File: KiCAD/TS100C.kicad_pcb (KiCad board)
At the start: 4 copper layers, 84 x 10 mm, 63 parts, among them J1 USB_C_Receptacle_USB2.0, J2 OLED_64x32, J3 A, J4 B, J5 DNP, P1 TC2030-CTX, Q1 SS8050, Q2 DMP3017SFG, SW1 key1, SW2 key2, U1 USBLC6-4SC6, U2 AP2204R-3.3, U3 STUSB4500, U4 STM32F072C8Ux, U5 OPA340NA, U6 MCP9700AT-ETT, U7 SI8540

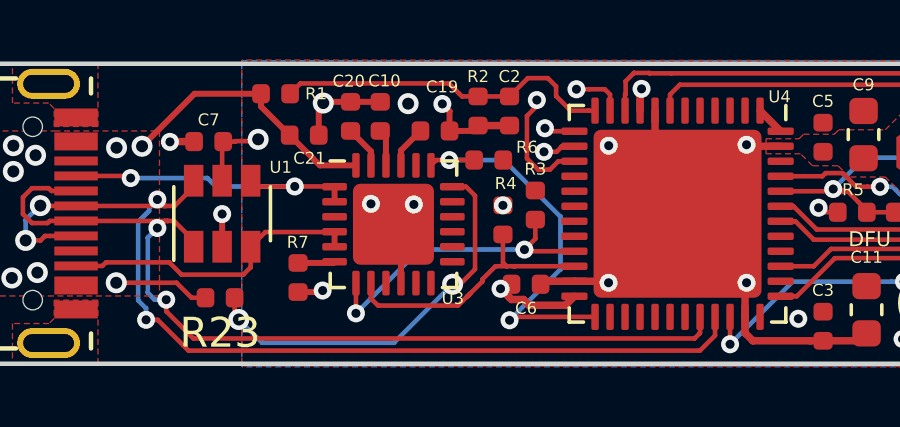
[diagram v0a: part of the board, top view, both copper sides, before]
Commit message: updated hardware
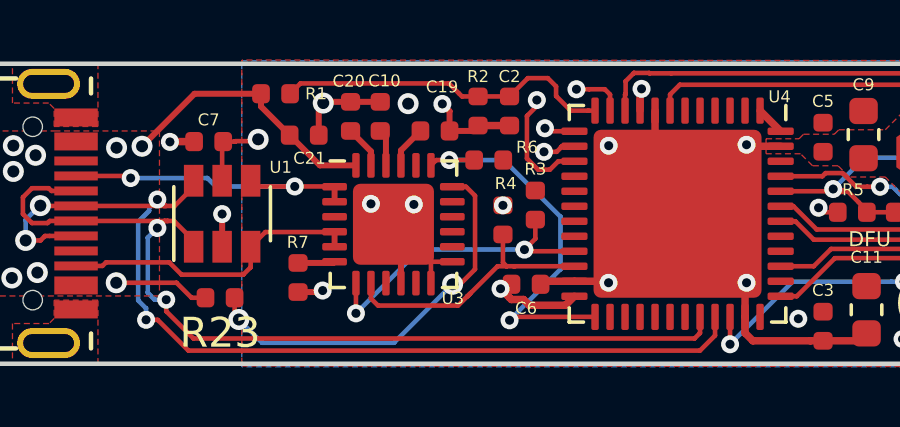
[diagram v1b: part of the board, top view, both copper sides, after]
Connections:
- U3 pad 12: Net-(U3-Pad12) -> GND
- U3 pad 13: Net-(U3-Pad13) -> GND
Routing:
- net GND: track 56.5 -> 59.7 mm
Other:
- rule pad_to_mask_clearance: 0.154 -> 0.1
- rule solder_mask_min_width: 0.25 -> 0.154

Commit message: added todos
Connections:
- U4 pad 29: Net-(U4-Pad29) -> PWM
- U4 pad 39: PWM -> Net-(U4-Pad39)
